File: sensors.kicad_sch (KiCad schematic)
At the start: 10 parts, among them U10 BHI360, U21 PCA9517DP,118, U26 BME680

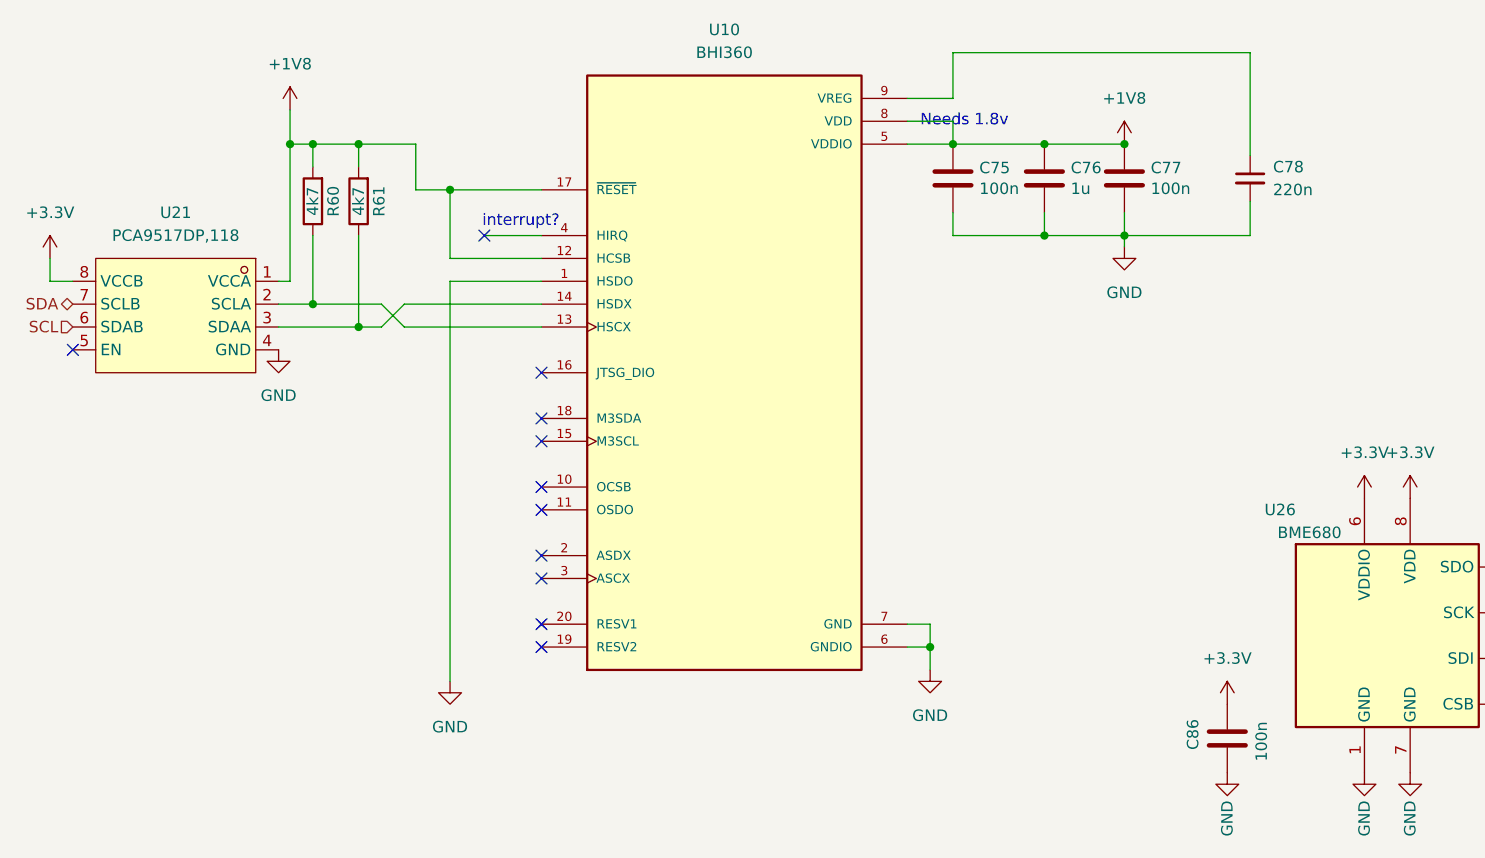
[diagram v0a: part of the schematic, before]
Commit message: Add ESD protection to USB ports, remove fuse from USB-C port, small fixes
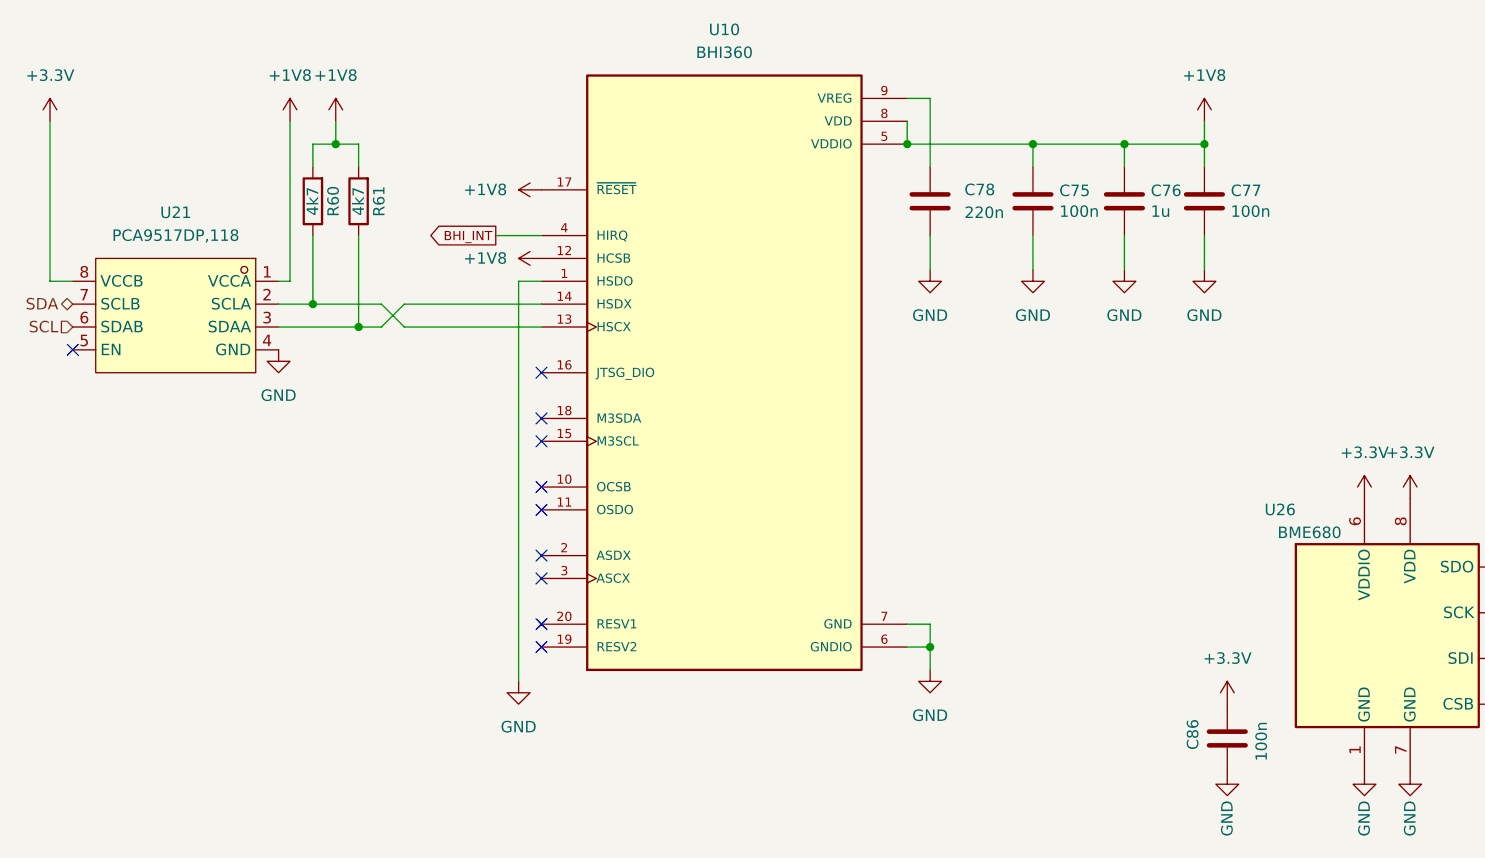
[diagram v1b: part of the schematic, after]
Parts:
- C78: symbol Device:C_Small -> Device:C
- U10: Availability In Stock -> (none); Check_prices https://www.snapeda.com/parts/BHI360/Bosch/view-part/?ref=e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 -> (none); Description_1 Multiple Function Sensor Development Tools Multiple Functio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 -> (none); MANUFACTURER Bosch Sensortec -> (none); MP BHI360 -> (none); PARTREV 1.0 -> (none); Price None -> (none); STANDARD Manufacturer Recommendations -> (none); SnapEDA_Link https://www.snapeda.com/parts/BHI360/Bosch/view-part/?ref=s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 -> (none)
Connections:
- net BHI_INT: now reaches U10.4 (HIRQ)
- no-connect marks 11 -> 10
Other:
- note removed: "Needs 1.8v"
- note removed: "interrupt?"
- moved on the sheet: C75, C76, C77, C78

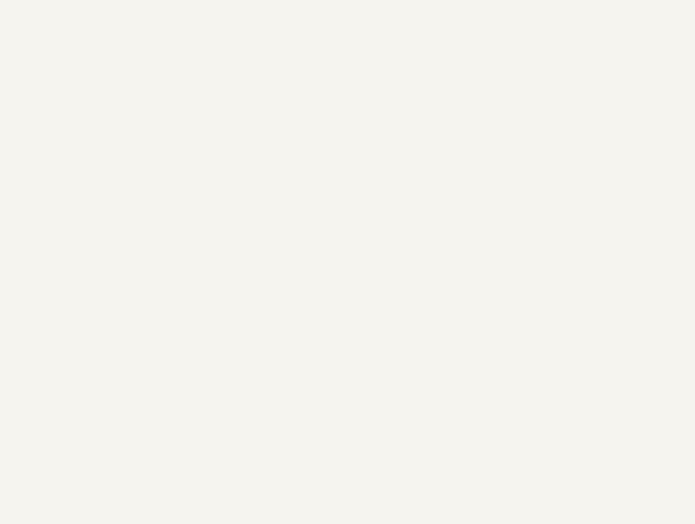
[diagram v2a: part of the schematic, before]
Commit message: Add accelerometer interrupt
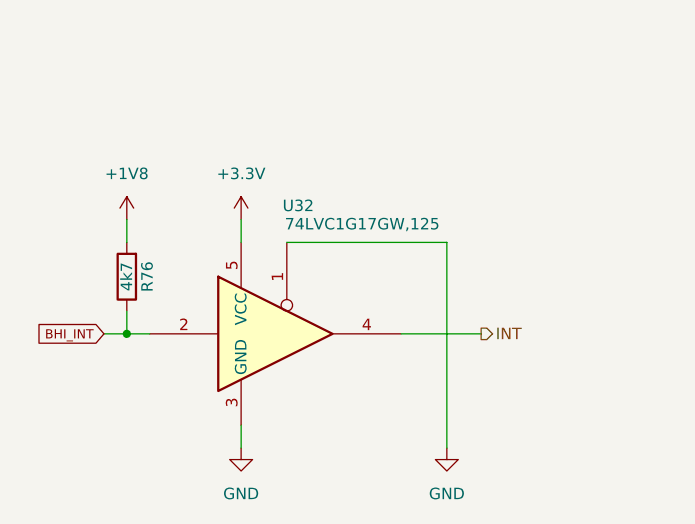
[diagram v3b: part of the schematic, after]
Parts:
- added R76: 4k7, Resistor_SMD:R_0402_1005Metric, symbol Device:R
- added U32: 74LVC1G17GW,125, Package_TO_SOT_SMD:SOT-353_SC-70-5, symbol 74xGxx:74LVC1G125
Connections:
- net +1V8: now also R76.2
- net +3.3V: now also U32.5 (VCC)
- net BHI_INT: now also R76.1, U32.2
- net GND: now also U32.1, U32.3 (GND)
- new net INT: U32.4

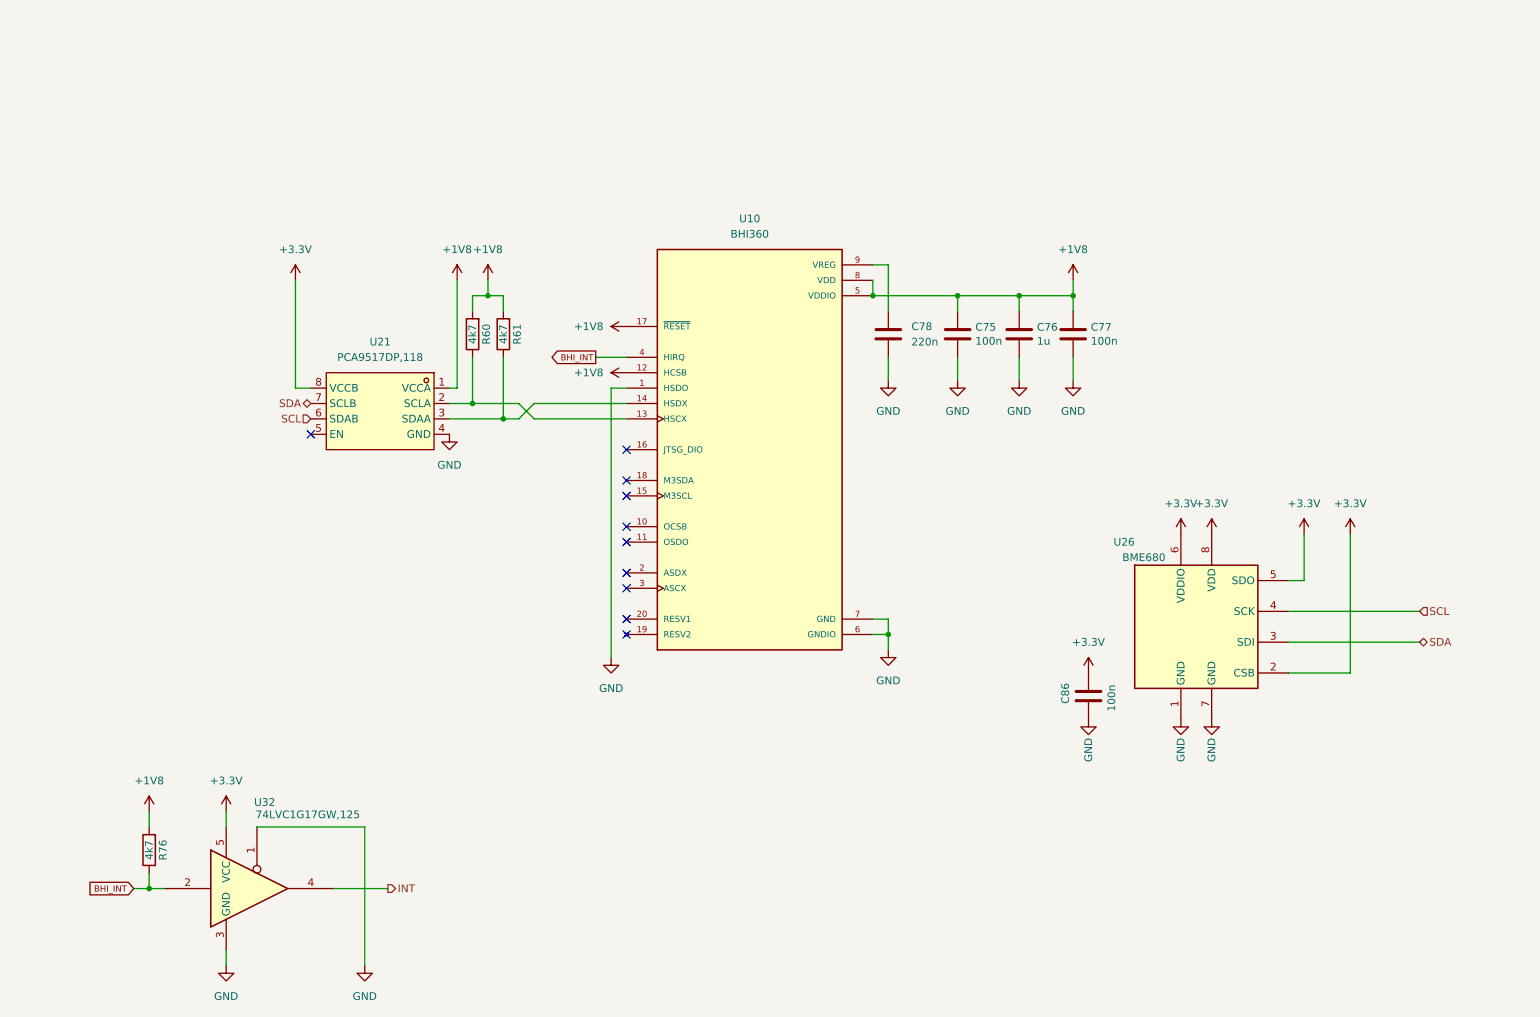
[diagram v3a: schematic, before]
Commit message: Add replace bme680 with bme688 on the design.
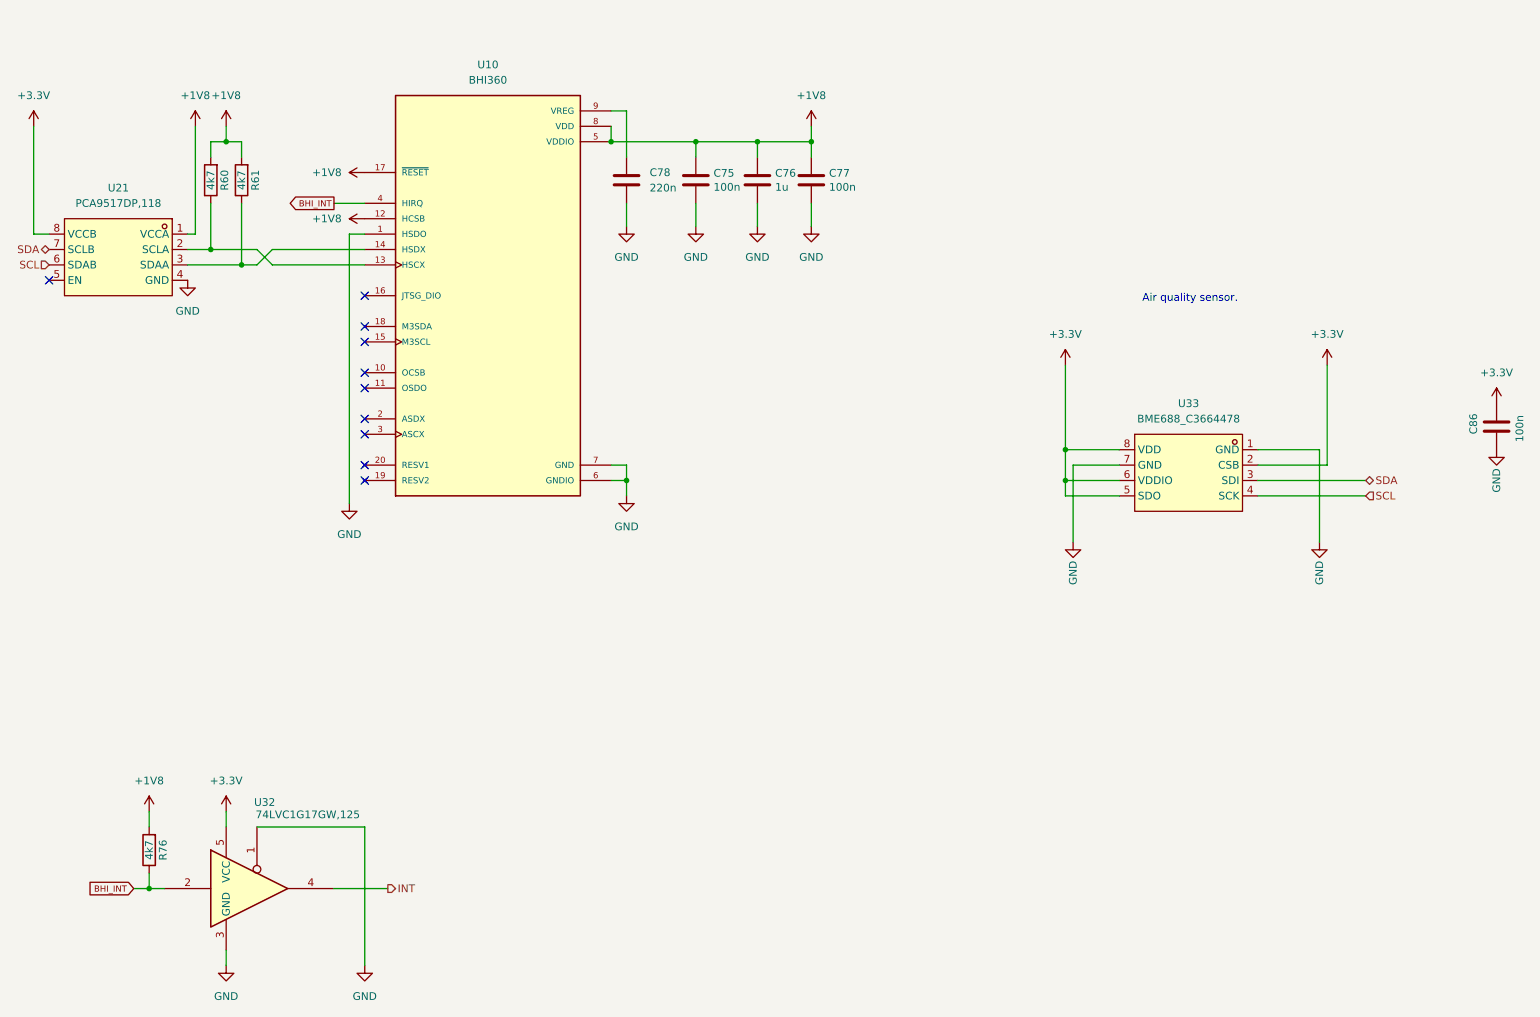
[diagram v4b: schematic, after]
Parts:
- removed U26: BME680, Package_LGA:Bosch_LGA-8_3x3mm_P0.8mm_ClockwisePinNumbering, symbol mch2021-rescue:BME680-Sensor
- added U33: BME688_C3664478, lcsc:LGA-8_L3.0-W3.0-P0.80_BME688, symbol lcsc:BME688_C3664478
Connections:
- net +3.3V: now also U33.2 (CSB), U33.5 (SDO), U33.6 (VDDIO), U33.8 (VDD)
- net GND: now also U33.1 (GND), U33.7 (GND)
- net SCL: now also U33.4 (SCK)
- net SDA: now also U33.3 (SDI)
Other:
- note added: "Air quality sensor."
- moved on the sheet: C75, C76, C77, C78, C86, R60, R61, U10, U21

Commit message: Add BMI270 sensor
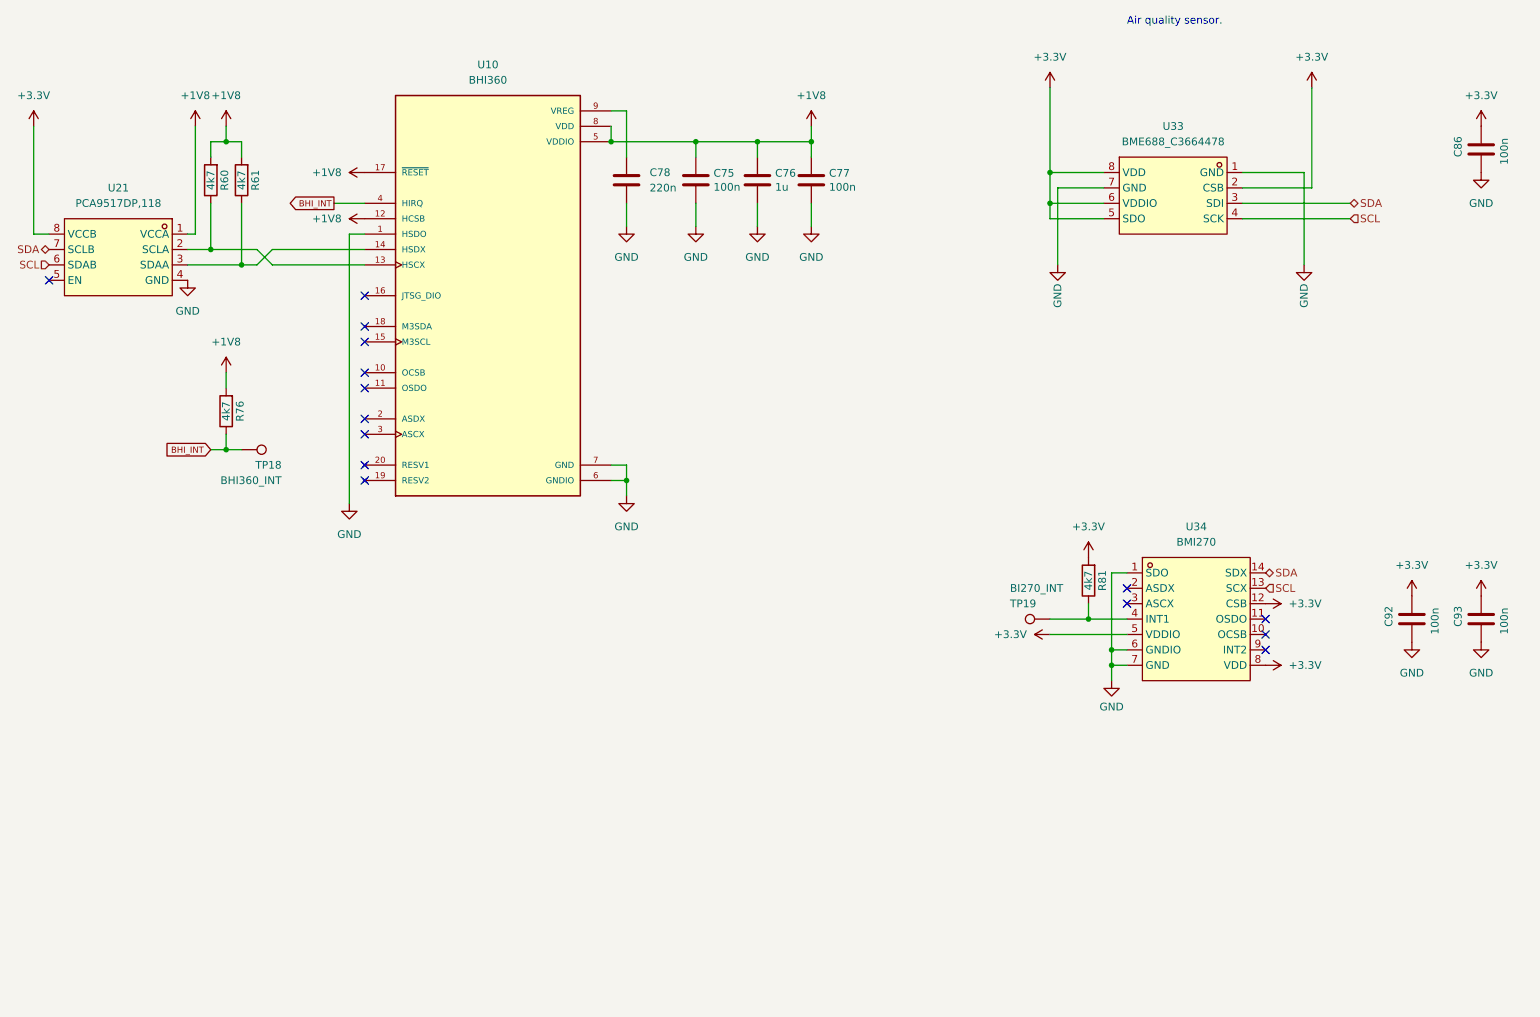
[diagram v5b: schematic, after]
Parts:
- removed U32: 74LVC1G17GW,125, Package_TO_SOT_SMD:SOT-353_SC-70-5, symbol 74xGxx:74LVC1G125
- added C92, C93: 100n, Capacitor_SMD:C_0402_1005Metric, symbol mch2021-rescue:C-Device
- added R81: 4k7, Resistor_SMD:R_0402_1005Metric, symbol Device:R
- added TP18: BHI360_INT, TestPoint:TestPoint_Pad_D1.0mm, symbol Connector:TestPoint
- added TP19: BI270_INT, TestPoint:TestPoint_Pad_D1.0mm, symbol Connector:TestPoint
- added U34: BMI270, library:LGA-14_L3.0-W2.5-P0.50-BR, symbol BMI270:BMI270
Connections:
- net +3.3V: now also C92.1, C93.1, R81.2, U34.12 (CSB), U34.5 (VDDIO), U34.8 (VDD)
- net BHI_INT: now also TP18.1
- net GND: now also C92.2, C93.2, U34.1 (SDO), U34.6 (GNDIO), U34.7 (GND)
- net SCL: now also U34.13 (SCX)
- net SDA: now also U34.14 (SDX)
- new net: R81.1, TP19.1, U34.4 (INT1)
- no-connect marks 10 -> 15
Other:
- moved on the sheet: C86, R76, U33
